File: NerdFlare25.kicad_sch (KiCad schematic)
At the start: 31 parts, among them J1 VEXT, SW1 SW_Push, SW2 SW_SPDT, T1 DMG2305

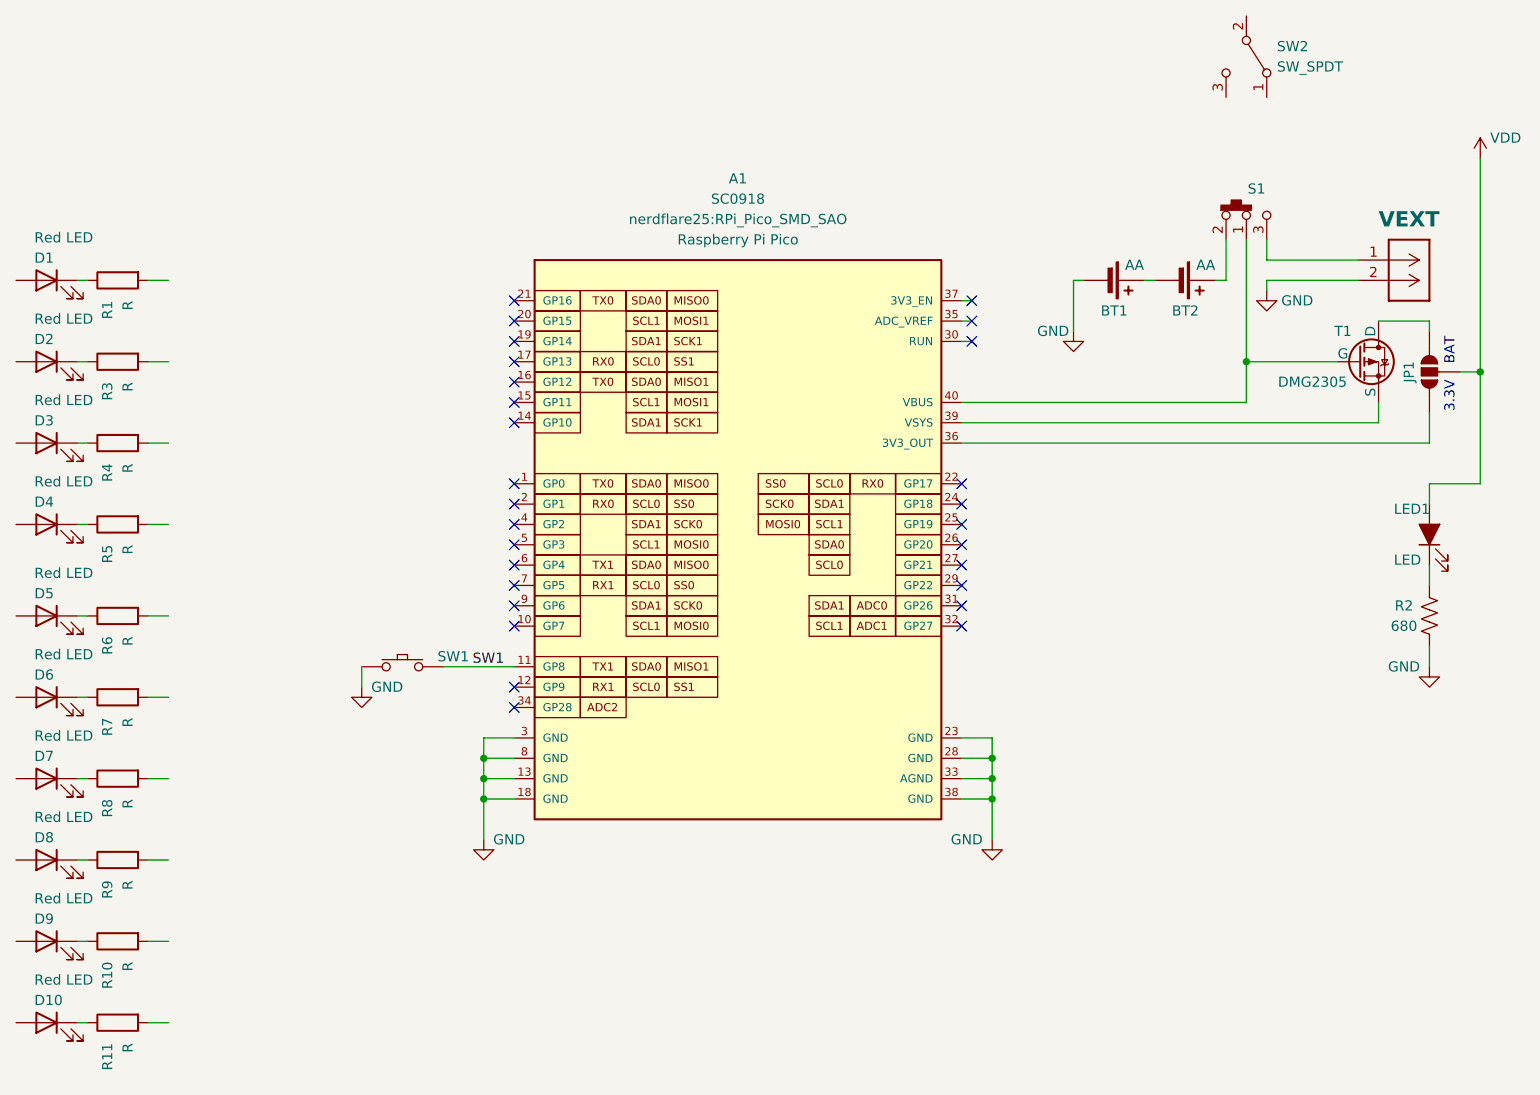
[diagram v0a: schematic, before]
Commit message: This is v0; going to fab.
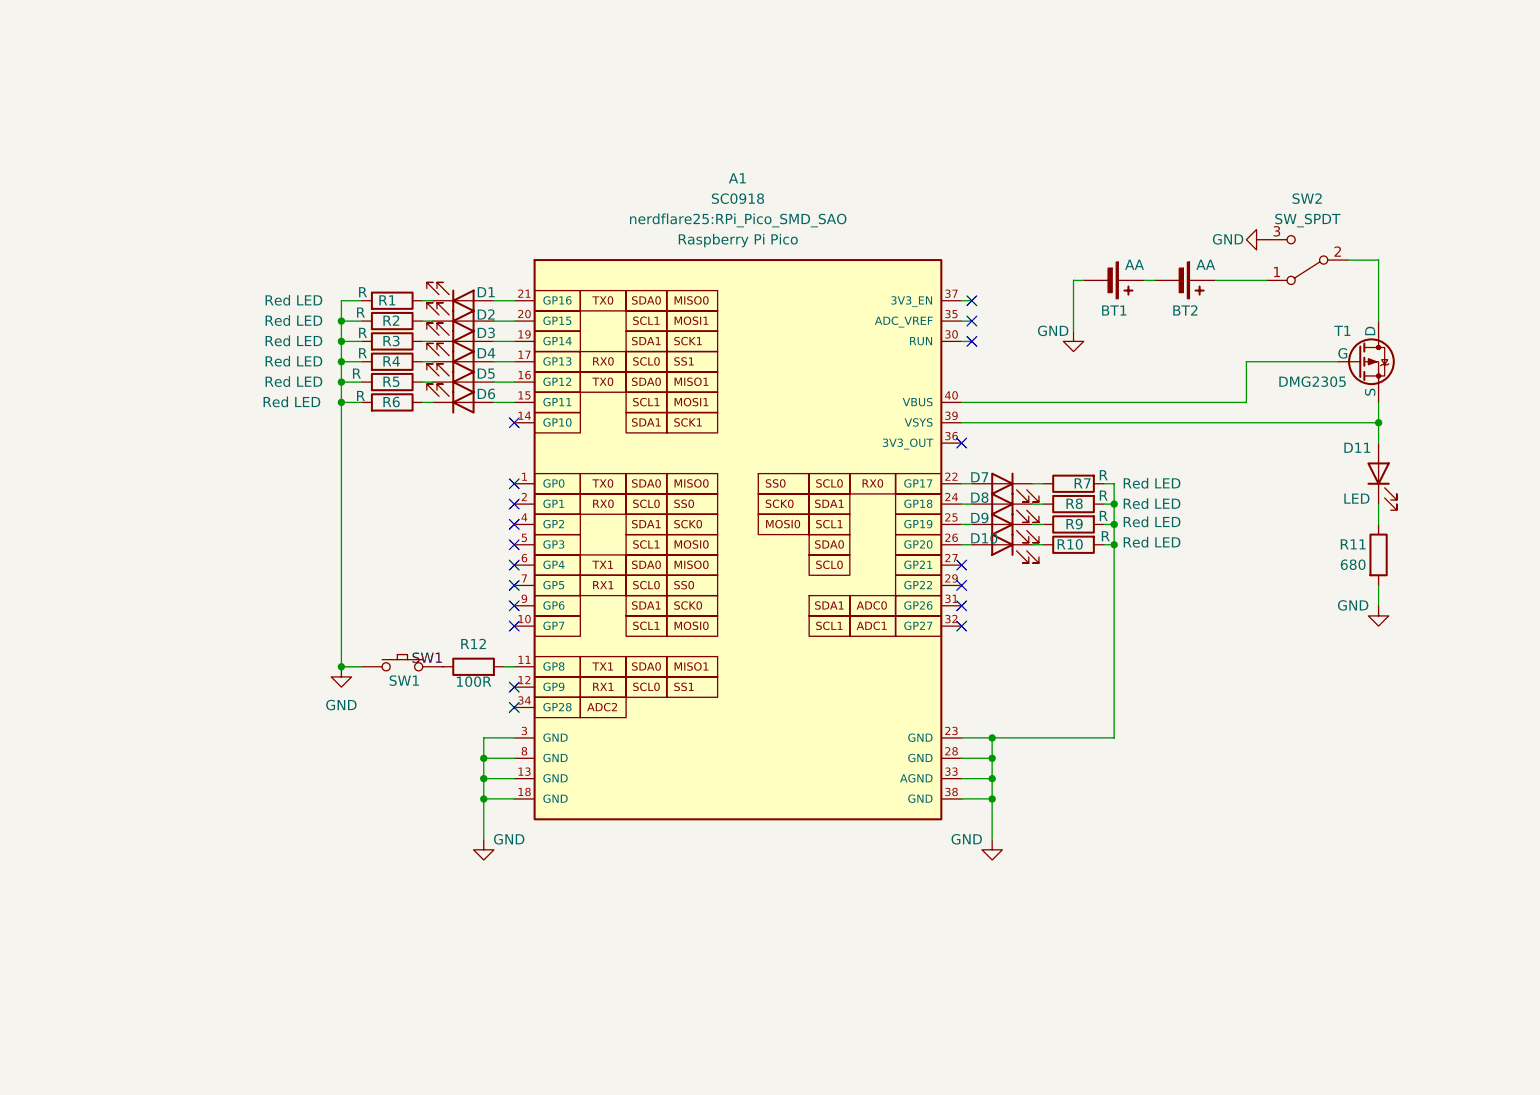
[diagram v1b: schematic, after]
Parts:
- removed J1: VEXT, nerdflare25:SAO_PinHeader_1x02_P2.54mm_SMD, symbol .badge24:IO_JACK_M02
- removed JP1: SolderJumper_3_Open, nerdflare25:SolderJumper_Open_Rounded_SAO, symbol .badge24:SolderJumper_3_Open
- removed S1: SW_Slide_SPDT, nerdflare25:SW_Slide-03_Wuerth-WS-SLTV_10x2.5x6.4_P2.54mm, symbol .badge24:SW_Slide_SPDT_SMALL
- added R12: 100R, Resistor_SMD:R_1206_3216Metric_Pad1.30x1.75mm_HandSolder, symbol Device:R
- D11: renamed from LED1; symbol .badge24:LED -> Device:LED
- R11: renamed from R2; symbol .badge24:RES -> Device:R
- renumbered D10 to D1, D6 to D10, D1 to D2, D2 to D3, D3 to D4, D4 to D5, D5 to D6, D9 to D7, D7 to D9, R11 to R1, R7 to R10, R1 to R2, R10 to R7, R9 to R8, R8 to R9
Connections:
- net VDD is gone; now on an unnamed net: D11.2 (A)
- net GND: now also R1.2, R10.2, R2.2, R3.2, R4.2, R5.2, R6.2, R7.2, R8.2, R9.2, SW2.3 (C)
- net SW1: now also R12.1; no longer A1.11 (GP8)
- net at T1.3 (D): now also SW2.2 (B)
- net at BT2.1 (+): now also SW2.1 (A)
- net at D7.2 (A): now also A1.22 (GP17)
- net at D6.2 (A): now also A1.15 (GP11)
- net at D8.2 (A): now also A1.24 (GP18)
- net at D2.2 (A): now also A1.20 (GP15)
- net at D5.2 (A): now also A1.16 (GP12)
- net at D4.2 (A): now also A1.17 (GP13)
- net at D9.2 (A): now also A1.25 (GP19)
- net at D3.2 (A): now also A1.19 (GP14)
- net at A1.21 (GP16): now also D1.2 (A)
- net at A1.26 (GP20): now also D10.2 (A)
- new net: A1.11 (GP8), R12.2
- no-connect marks 28 -> 19
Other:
- note removed: "3.3V"
- note removed: "BAT"
- moved on the sheet: D1, D10, D2, D3, D4, D5, D6, D7, D8, D9, R1, R10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
